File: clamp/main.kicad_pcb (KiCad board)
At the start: 2 copper layers, 78 parts, among them P1 CONN_01X12, P2 CONN_01X15, P3 CONN_01X03, P4 CONN_01X06, Q1 2N3904, U1 LM741, U12 LTZ1000, U13 LM741, U14 LM741, U2 LM741, U3 LM741, U4 LM741, U5 LM741, U6 LM741, U7 LM741

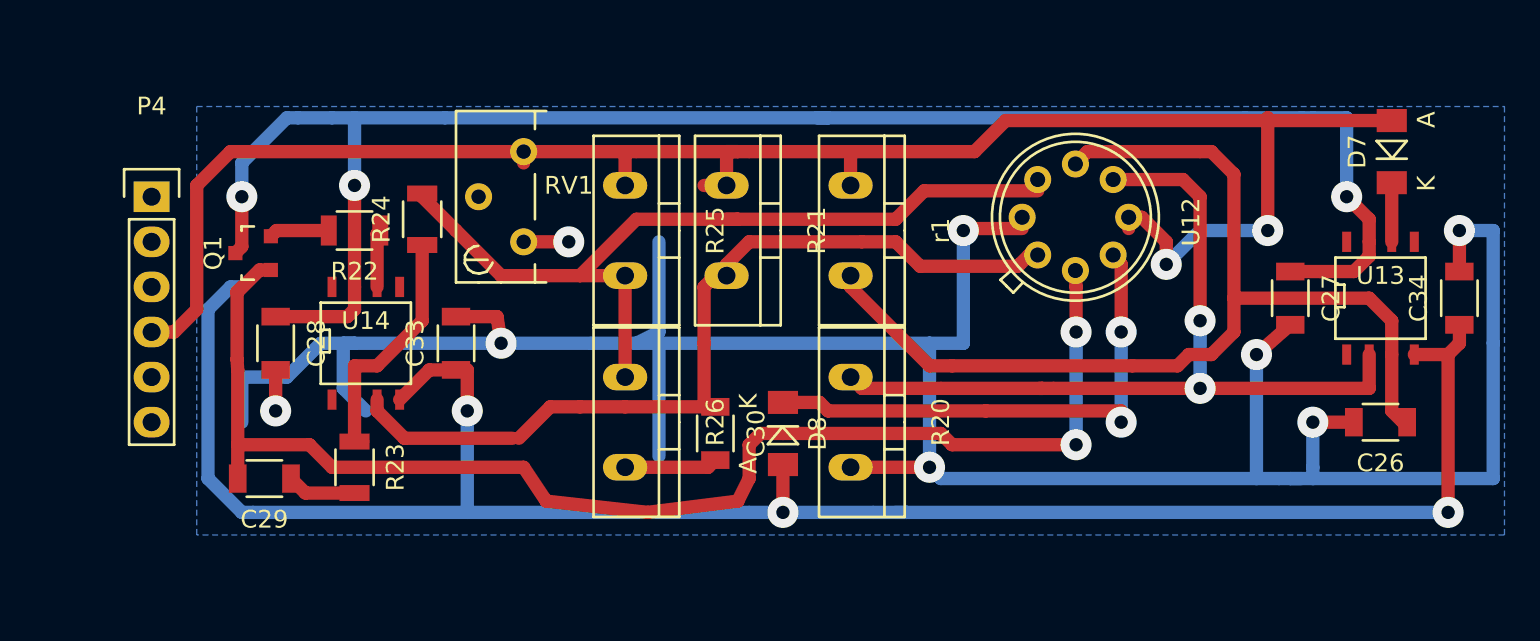
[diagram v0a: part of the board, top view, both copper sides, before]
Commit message: update
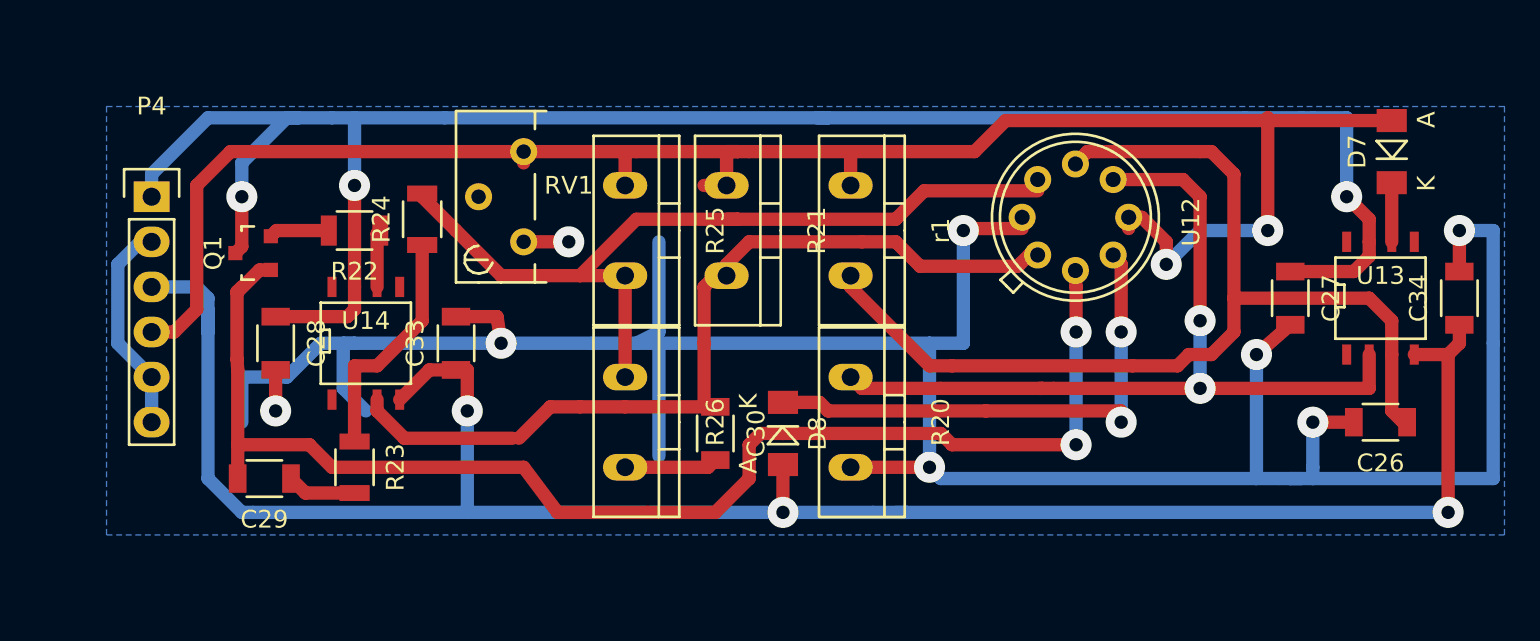
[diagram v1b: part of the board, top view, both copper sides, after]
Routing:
- net GND: track 207.6 -> 219.7 mm
- net +VE: track 380.8 -> 391.7 mm
- net -VE: track 362.7 -> 365.7 mm
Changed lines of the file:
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@@
   (general
     (links 171)
-    (no_connects 87)
+    (no_connects 82)
     (area -5.909001 -6.355 253.23 151.352002)
     (thickness 1.6)
     (drawings 13)
-    (tracks 524)
+    (tracks 534)
     (zones 0)
     (modules 78)
@@
     (effects (font (size 1.5 1.5) (thickness 0.3)))
   )
+  (segment (start 184.15 40.005) (end 179.07 40.005) (width 0.75) (layer B.Cu) (net 1))
+  (segment (start 175.895 43.18) (end 175.895 44.45) (width 0.75) (layer B.Cu) (net 1))
+  (segment (start 179.07 40.005) (end 175.895 43.18) (width 0.75) (layer B.Cu) (net 1))
   (segment (start 187.325 40.005) (end 187.325 43.815) (width 0.75) (layer B.Cu) (net 1))
   (via (at 187.325 43.815) (size 1.75) (drill 0.75) (layers F.Cu B.Cu) (net 1))
@@
   (via (at 121.92 86.36) (size 1.75) (drill 0.75) (layers F.Cu B.Cu) (net 1))
   (segment (start 121.92 86.36) (end 166.624 86.36) (width 0.75) (layer B.Cu) (net 1))
+  (segment (start 179.07 52.07) (end 179.07 50.165) (width 0.75) (layer B.Cu) (net 2))
+  (segment (start 178.435 49.53) (end 175.895 49.53) (width 0.75) (layer B.Cu) (net 2))
+  (segment (start 179.07 50.165) (end 178.435 49.53) (width 0.75) (layer B.Cu) (net 2))
   (segment (start 193.675 62.23) (end 193.675 56.515) (width 0.75) (layer B.Cu) (net 2))
   (via (at 193.675 56.515) (size 1.75) (drill 0.75) (layers F.Cu B.Cu) (net 2))
   (segment (start 193.675 56.515) (end 193.675 54.205) (width 0.75) (layer F.Cu) (net 2))
-  (segment (start 180.975 49.53) (end 180.34 49.53) (width 0.75) (layer B.Cu) (net 2))
-  (segment (start 180.34 49.53) (end 179.07 50.8) (width 0.75) (layer B.Cu) (net 2))
-  (segment (start 179.07 50.8) (end 179.07 60.325) (width 0.75) (layer B.Cu) (net 2))
+  (segment (start 179.07 50.8) (end 179.07 52.07) (width 0.75) (layer B.Cu) (net 2))
+  (segment (start 179.07 52.07) (end 179.07 60.325) (width 0.75) (layer B.Cu) (net 2))
   (segment (start 179.07 60.325) (end 180.975 62.23) (width 0.75) (layer B.Cu) (net 2))
   (segment (start 180.975 62.23) (end 181.61 62.23) (width 0.75) (layer B.Cu) (net 2))
-  (segment (start 198.755 62.23) (end 193.675 62.23) (width 0.75) (layer B.Cu) (net 2))
+  (segment (start 207.01 62.23) (end 193.675 62.23) (width 0.75) (layer B.Cu) (net 2))
   (segment (start 193.675 62.23) (end 181.61 62.23) (width 0.75) (layer B.Cu) (net 2))
-  (segment (start 209.55 62.23) (end 198.755 62.23) (width 0.75) (layer B.Cu) (net 2))
+  (segment (start 208.28 62.23) (end 207.01 62.23) (width 0.75) (layer B.Cu) (net 2))
   (segment (start 248.92 53.34) (end 248.92 62.23) (width 0.75) (layer F.Cu) (net 2))
   (via (at 248.92 62.23) (size 1.75) (drill 0.75) (layers F.Cu B.Cu) (net 2))
@@
   (segment (start 249.555 52.705) (end 249.555 51.665) (width 0.75) (layer F.Cu) (net 2))
   (segment (start 248.92 53.34) (end 249.555 52.705) (width 0.75) (layer F.Cu) (net 2))
-  (segment (start 211.455 62.23) (end 209.55 62.23) (width 0.75) (layer B.Cu) (net 2))
+  (segment (start 211.455 62.23) (end 208.28 62.23) (width 0.75) (layer B.Cu) (net 2))
   (segment (start 193.675 54.205) (end 191.54 54.205) (width 0.75) (layer F.Cu) (net 2))
   (segment (start 191.54 54.205) (end 189.865 55.88) (width 0.75) (layer F.Cu) (net 2))
@@
   (segment (start 165.862 96.012) (end 165.862 96.52) (width 0.75) (layer B.Cu) (net 2))
   (segment (start 157.132 104.775) (end 160.30194 104.648) (width 0.75) (layer F.Cu) (net 3) (status 30))
+  (segment (start 175.895 46.99) (end 175.26 46.99) (width 0.75) (layer B.Cu) (net 4))
+  (segment (start 175.26 46.99) (end 173.99 48.26) (width 0.75) (layer B.Cu) (net 4))
+  (segment (start 173.99 48.26) (end 173.99 52.705) (width 0.75) (layer B.Cu) (net 4))
+  (segment (start 173.99 52.705) (end 175.895 54.61) (width 0.75) (layer B.Cu) (net 4))
+  (segment (start 175.895 57.15) (end 175.895 54.61) (width 0.75) (layer B.Cu) (net 4))
   (segment (start 202.565 59.69) (end 207.24 59.69) (width 0.75) (layer F.Cu) (net 4))
   (segment (start 207.24 59.69) (end 207.645 59.285) (width 0.75) (layer F.Cu) (net 4))
@@
   (segment (start 217.805 45.72) (end 208.915 45.72) (width 0.75) (layer F.Cu) (net 33))
   (segment (start 191.135 44.45) (end 191.135 44.27) (width 0.75) (layer F.Cu) (net 33))
+  (segment (start 207.645 62.23) (end 209.55 60.325) (width 0.75) (layer F.Cu) (net 34))
+  (segment (start 227.965 58.42) (end 220.98 58.42) (width 0.75) (layer F.Cu) (net 34))
+  (via (at 227.965 52.07) (size 1.75) (drill 0.75) (layers F.Cu B.Cu) (net 34))
+  (segment (start 227.965 58.42) (end 227.965 52.07) (width 0.75) (layer B.Cu) (net 34))
+  (via (at 227.965 58.42) (size 1.75) (drill 0.75) (layers F.Cu B.Cu) (net 34))
+  (segment (start 209.55 60.325) (end 209.55 58.42) (width 0.75) (layer F.Cu) (net 34))
+  (segment (start 209.55 58.42) (end 210.185 57.785) (width 0.75) (layer F.Cu) (net 34))
+  (segment (start 210.185 57.785) (end 211.455 57.785) (width 0.75) (layer F.Cu) (net 34))
+  (segment (start 220.345 57.785) (end 211.455 57.785) (width 0.75) (layer F.Cu) (net 34))
+  (segment (start 220.98 58.42) (end 220.345 57.785) (width 0.75) (layer F.Cu) (net 34))
   (segment (start 182.61076 48.575) (end 181.97576 48.575) (width 0.75) (layer F.Cu) (net 34))
   (segment (start 181.97576 48.575) (end 180.70576 49.845) (width 0.75) (layer F.Cu) (net 34))
@@
   (segment (start 180.745 54.205) (end 180.745 58.42) (width 0.75) (layer F.Cu) (net 34))
   (segment (start 180.70576 53.60924) (end 180.745 54.205) (width 0.75) (layer F.Cu) (net 34))
-  (segment (start 203.835 62.23) (end 208.915 61.595) (width 0.75) (layer F.Cu) (net 34))
+  (segment (start 203.835 62.23) (end 207.645 62.23) (width 0.75) (layer F.Cu) (net 34))
   (segment (start 180.745 58.42) (end 184.785 58.42) (width 0.75) (layer F.Cu) (net 34))
-  (segment (start 208.915 61.595) (end 209.55 60.325) (width 0.75) (layer F.Cu) (net 34))
-  (segment (start 198.12 61.595) (end 203.835 62.23) (width 0.75) (layer F.Cu) (net 34))
-  (segment (start 196.85 59.69) (end 198.12 61.595) (width 0.75) (layer F.Cu) (net 34))
+  (segment (start 198.755 62.23) (end 203.835 62.23) (width 0.75) (layer F.Cu) (net 34))
+  (segment (start 196.85 59.69) (end 198.755 62.23) (width 0.75) (layer F.Cu) (net 34))
   (segment (start 186.055 59.69) (end 196.85 59.69) (width 0.75) (layer F.Cu) (net 34))
   (segment (start 184.785 58.42) (end 186.055 59.69) (width 0.75) (layer F.Cu) (net 34))
   (segment (start 180.745 58.42) (end 180.745 60.325) (width 0.75) (layer F.Cu) (net 34))
-  (segment (start 220.98 58.42) (end 220.345 57.785) (width 0.75) (layer F.Cu) (net 34))
-  (segment (start 220.345 57.785) (end 211.455 57.785) (width 0.75) (layer F.Cu) (net 34))
-  (segment (start 210.185 57.785) (end 211.455 57.785) (width 0.75) (layer F.Cu) (net 34))
-  (segment (start 209.55 58.42) (end 210.185 57.785) (width 0.75) (layer F.Cu) (net 34))
-  (segment (start 209.55 60.325) (end 209.55 58.42) (width 0.75) (layer F.Cu) (net 34))
-  (via (at 227.965 58.42) (size 1.75) (drill 0.75) (layers F.Cu B.Cu) (net 34))
-  (segment (start 227.965 58.42) (end 227.965 52.07) (width 0.75) (layer B.Cu) (net 34))
-  (via (at 227.965 52.07) (size 1.75) (drill 0.75) (layers F.Cu B.Cu) (net 34))
-  (segment (start 227.965 58.42) (end 220.98 58.42) (width 0.75) (layer F.Cu) (net 34))
   (segment (start 227.9275 48.6075) (end 227.9275 48.9325) (width 0.75) (layer F.Cu) (net 34) (status 30))
   (segment (start 227.9275 48.9325) (end 227.965 49.53) (width 0.75) (layer F.Cu) (net 34) (status 10))
@@
     (polygon
       (pts
-        (xy 252.095 63.5) (xy 178.435 63.5) (xy 178.435 39.37) (xy 252.095 39.37)
+        (xy 252.095 63.5) (xy 173.355 63.5) (xy 173.355 39.37) (xy 252.095 39.37)
       )
     )
